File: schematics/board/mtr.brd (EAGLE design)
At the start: 19 x 13 mm, 11 parts

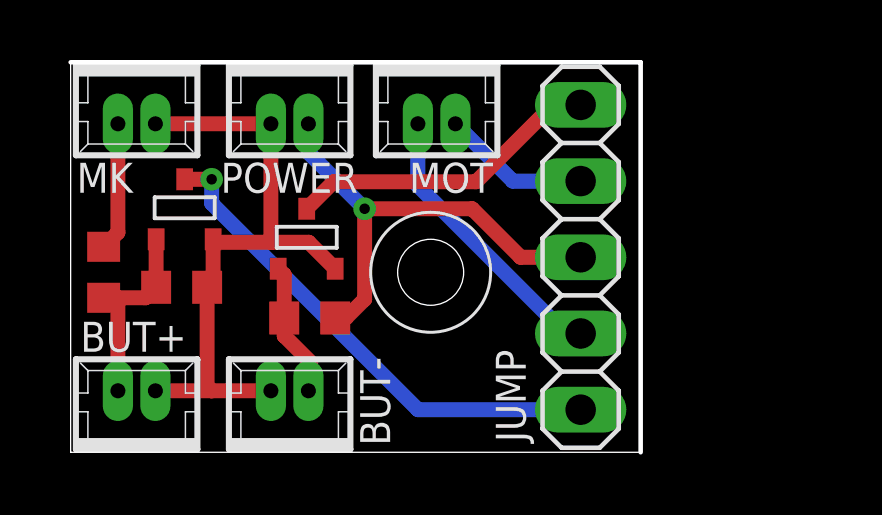
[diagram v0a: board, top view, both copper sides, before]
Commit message: Подготовлены платы SP и mtr
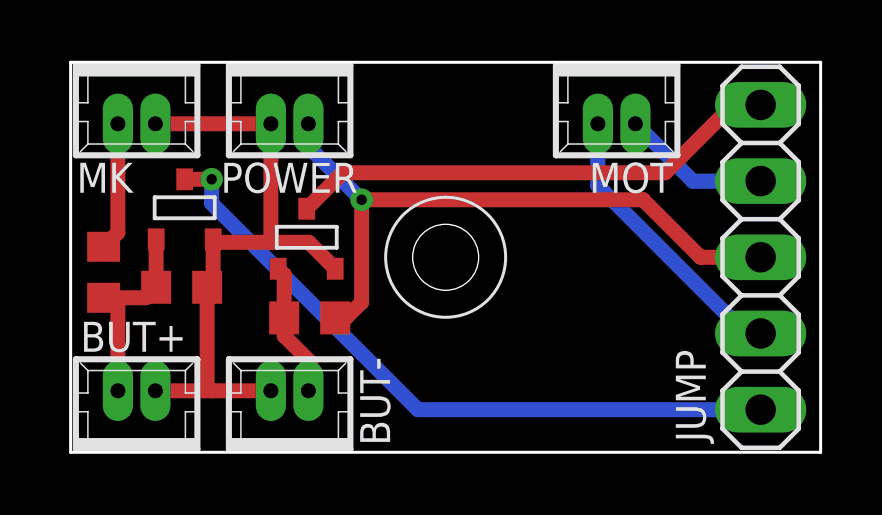
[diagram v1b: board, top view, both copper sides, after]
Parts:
- moved JUMP 6.00 mm to (23.0, 6.50)
- moved MOT 6.00 mm to (18.2, 11.4)
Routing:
- net 12V: track 15.7 -> 21.9 mm
- net MOTOR3-G: track 16.8 -> 22.8 mm
- net MOTOR3+G: track 10.6 -> 16.6 mm
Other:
- board size 19 x 13 mm -> 25 x 13 mm
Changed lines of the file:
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@@
 <board>
 <plain>
-<wire x1="0" y1="0" x2="19" y2="0" width="0" layer="20"/>
-<hole x="12" y="6" drill="2.2"/>
-<wire x1="0" y1="13" x2="0" y2="0" width="0" layer="20"/>
-<wire x1="0" y1="13" x2="19" y2="13" width="0.1524" layer="20"/>
-<wire x1="19" y1="13" x2="19" y2="0" width="0.1524" layer="20"/>
-<circle x="12" y="6" radius="2" width="0.1" layer="21"/>
+<wire x1="0" y1="0" x2="25" y2="0" width="0.1" layer="20"/>
+<hole x="12.5" y="6.5" drill="2.2"/>
+<wire x1="0" y1="13" x2="0" y2="0" width="0.1" layer="20"/>
+<wire x1="0" y1="13" x2="25" y2="13" width="0.1" layer="20"/>
+<wire x1="25" y1="13" x2="25" y2="0" width="0.1" layer="20"/>
+<circle x="12.5" y="6.5" radius="2" width="0.1" layer="21"/>
 </plain>
 <attributes>
@@
 </element>
 <element name="U$21" library="CanCubeSat" package="SOT23-3" value="SI2302CDS" x="7.869" y="7.117" smashed="yes"/>
-<element name="JUMP" library="pinhead" library_urn="urn:adsk.eagle:library:325" package="1X05" package3d_urn="urn:adsk.eagle:package:22469/2" value="" x="17" y="6.5" smashed="yes" rot="R90">
-<attribute name="NAME" x="15.1712" y="0.3438" size="1" layer="25" ratio="15" rot="R90"/>
-<attribute name="POPULARITY" value="69" x="17" y="6.5" size="1.778" layer="27" rot="R90" display="off"/>
-<attribute name="VALUE" x="20.175" y="1.42" size="1.27" layer="27" rot="R90"/>
+<element name="JUMP" library="pinhead" library_urn="urn:adsk.eagle:library:325" package="1X05" package3d_urn="urn:adsk.eagle:package:22469/2" value="" x="23" y="6.5" smashed="yes" rot="R90">
+<attribute name="NAME" x="21.1712" y="0.3438" size="1" layer="25" ratio="15" rot="R90"/>
+<attribute name="POPULARITY" value="69" x="23" y="6.5" size="1.778" layer="27" rot="R90" display="off"/>
+<attribute name="VALUE" x="26.175" y="1.42" size="1.27" layer="27" rot="R90"/>
 </element>
 <element name="U$1" library="CanCubeSat" package="SOT23-3" value="SI2302CDS" x="3.8" y="8.1" smashed="yes"/>
@@
 <attribute name="POPULARITY" value="0" x="2.2" y="11.4" size="1.778" layer="27" rot="R180" display="off"/>
 </element>
-<element name="MOT" library="con-molex" library_urn="urn:adsk.eagle:library:165" package="53047-02" package3d_urn="urn:adsk.eagle:package:8078511/1" value="53047-02" x="12.2" y="11.4" smashed="yes" rot="R180">
-<attribute name="MF" value="MOLEX" x="12.2" y="11.4" size="1.778" layer="27" rot="R180" display="off"/>
-<attribute name="MPN" value="53047-0210" x="12.2" y="11.4" size="1.778" layer="27" rot="R180" display="off"/>
-<attribute name="NAME" x="14.075" y="9.65" size="1" layer="25" ratio="15" rot="R180"/>
-<attribute name="OC_FARNELL" value="9733051" x="12.2" y="11.4" size="1.778" layer="27" rot="R180" display="off"/>
-<attribute name="OC_NEWARK" value="57H4701" x="12.2" y="11.4" size="1.778" layer="27" rot="R180" display="off"/>
-<attribute name="POPULARITY" value="0" x="12.2" y="11.4" size="1.778" layer="27" rot="R180" display="off"/>
+<element name="MOT" library="con-molex" library_urn="urn:adsk.eagle:library:165" package="53047-02" package3d_urn="urn:adsk.eagle:package:8078511/1" value="53047-02" x="18.2" y="11.4" smashed="yes" rot="R180">
+<attribute name="MF" value="MOLEX" x="18.2" y="11.4" size="1.778" layer="27" rot="R180" display="off"/>
+<attribute name="MPN" value="53047-0210" x="18.2" y="11.4" size="1.778" layer="27" rot="R180" display="off"/>
+<attribute name="NAME" x="20.075" y="9.65" size="1" layer="25" ratio="15" rot="R180"/>
+<attribute name="OC_FARNELL" value="9733051" x="18.2" y="11.4" size="1.778" layer="27" rot="R180" display="off"/>
+<attribute name="OC_NEWARK" value="57H4701" x="18.2" y="11.4" size="1.778" layer="27" rot="R180" display="off"/>
+<attribute name="POPULARITY" value="0" x="18.2" y="11.4" size="1.778" layer="27" rot="R180" display="off"/>
 </element>
 <element name="POWER" library="con-molex" library_urn="urn:adsk.eagle:library:165" package="53047-02" package3d_urn="urn:adsk.eagle:package:8078511/1" value="53047-02" x="7.3" y="11.4" smashed="yes" rot="R180">
@@
 <contactref element="U$21" pad="3"/>
 <contactref element="JUMP" pad="5"/>
-<wire x1="13.517" y1="9.017" x2="8.769" y2="9.017" width="0.5" layer="1"/>
-<wire x1="7.869" y1="8.117" x2="8.769" y2="9.017" width="0.5" layer="1"/>
-<wire x1="16.08" y1="11.58" x2="17" y2="11.58" width="0.5" layer="1"/>
-<wire x1="13.517" y1="9.017" x2="16.08" y2="11.58" width="0.5" layer="1"/>
+<wire x1="19.817" y1="9.317" x2="9.069" y2="9.317" width="0.5" layer="1"/>
+<wire x1="7.869" y1="8.117" x2="9.069" y2="9.317" width="0.5" layer="1"/>
+<wire x1="22.08" y1="11.58" x2="23" y2="11.58" width="0.5" layer="1"/>
+<wire x1="19.817" y1="9.317" x2="22.08" y2="11.58" width="0.5" layer="1"/>
 </signal>
 <signal name="12V">
@@
 <contactref element="JUMP" pad="3"/>
 <contactref element="POWER" pad="2"/>
-<wire x1="17" y1="6.5" x2="15" y2="6.5" width="0.5" layer="1"/>
-<wire x1="13.383" y1="8.117" x2="9.8" y2="8.117" width="0.5" layer="1"/>
-<wire x1="9.8" y1="8.117" x2="9.8" y2="5.1" width="0.5" layer="1"/>
-<wire x1="9.8" y1="5.1" x2="9.177" y2="4.477" width="0.5" layer="1"/>
+<wire x1="23" y1="6.5" x2="21" y2="6.5" width="0.5" layer="1"/>
+<wire x1="19.083" y1="8.417" x2="9.7" y2="8.417" width="0.5" layer="1"/>
+<wire x1="9.7" y1="8.417" x2="9.7" y2="5" width="0.5" layer="1"/>
+<wire x1="9.7" y1="5" x2="9.177" y2="4.477" width="0.5" layer="1"/>
 <wire x1="8.819" y1="4.477" x2="9.177" y2="4.477" width="0.5" layer="1"/>
-<wire x1="15" y1="6.5" x2="13.383" y2="8.117" width="0.5" layer="1"/>
-<wire x1="7.925" y1="10.95" x2="7.925" y2="9.992" width="0.5" layer="16"/>
-<wire x1="7.925" y1="9.992" x2="9.8" y2="8.117" width="0.5" layer="16"/>
-<via x="9.8" y="8.117" extent="1-16" drill="0.35"/>
+<wire x1="21" y1="6.5" x2="19.083" y2="8.417" width="0.5" layer="1"/>
+<wire x1="7.925" y1="10.95" x2="7.925" y2="10.192" width="0.5" layer="16"/>
+<wire x1="7.925" y1="10.192" x2="9.7" y2="8.417" width="0.5" layer="16"/>
+<via x="9.7" y="8.417" extent="1-16" drill="0.35"/>
 </signal>
 <signal name="MOTOR3+">
 <contactref element="JUMP" pad="4"/>
 <contactref element="MOT" pad="2"/>
-<wire x1="17" y1="9.04" x2="14.735" y2="9.04" width="0.5" layer="16"/>
-<wire x1="14.735" y1="9.04" x2="12.825" y2="10.95" width="0.5" layer="16"/>
+<wire x1="23" y1="9.04" x2="20.735" y2="9.04" width="0.5" layer="16"/>
+<wire x1="20.735" y1="9.04" x2="18.825" y2="10.95" width="0.5" layer="16"/>
 </signal>
 <signal name="MOTOR3-">
 <contactref element="JUMP" pad="2"/>
 <contactref element="MOT" pad="1"/>
-<wire x1="17" y1="3.96" x2="16.5" y2="3.96" width="0.5" layer="16"/>
-<wire x1="16.5" y1="3.96" x2="11.575" y2="8.885" width="0.5" layer="16"/>
-<wire x1="11.575" y1="8.885" x2="11.575" y2="10.95" width="0.5" layer="16"/>
+<wire x1="23" y1="3.96" x2="22.5" y2="3.96" width="0.5" layer="16"/>
+<wire x1="22.5" y1="3.96" x2="17.575" y2="8.885" width="0.5" layer="16"/>
+<wire x1="17.575" y1="8.885" x2="17.575" y2="10.95" width="0.5" layer="16"/>
 </signal>
 <signal name="N$17">
@@
 <wire x1="11.58" y1="1.42" x2="4.7" y2="8.3" width="0.5" layer="16"/>
 <wire x1="4.7" y1="9.1" x2="4.7" y2="8.3" width="0.5" layer="16"/>
-<wire x1="11.58" y1="1.42" x2="17" y2="1.42" width="0.5" layer="16"/>
+<wire x1="11.58" y1="1.42" x2="23" y2="1.42" width="0.5" layer="16"/>
 </signal>
 </signals>
